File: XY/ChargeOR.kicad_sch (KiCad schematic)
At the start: 8 parts, among them U13 LTC4376CDHD_PBF, U9 SI3865DDV-T1-GE3

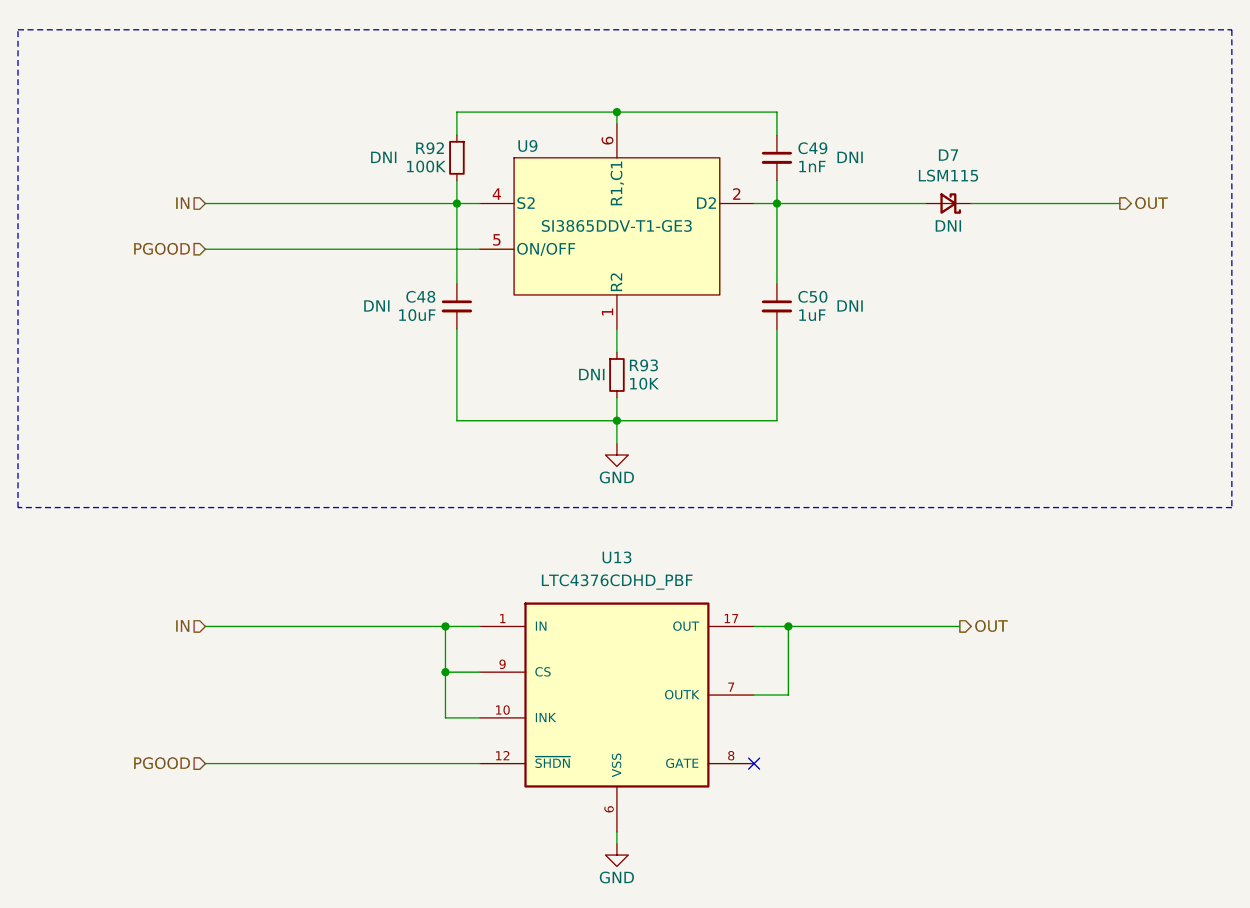
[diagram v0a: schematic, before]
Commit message: Updated XY boards
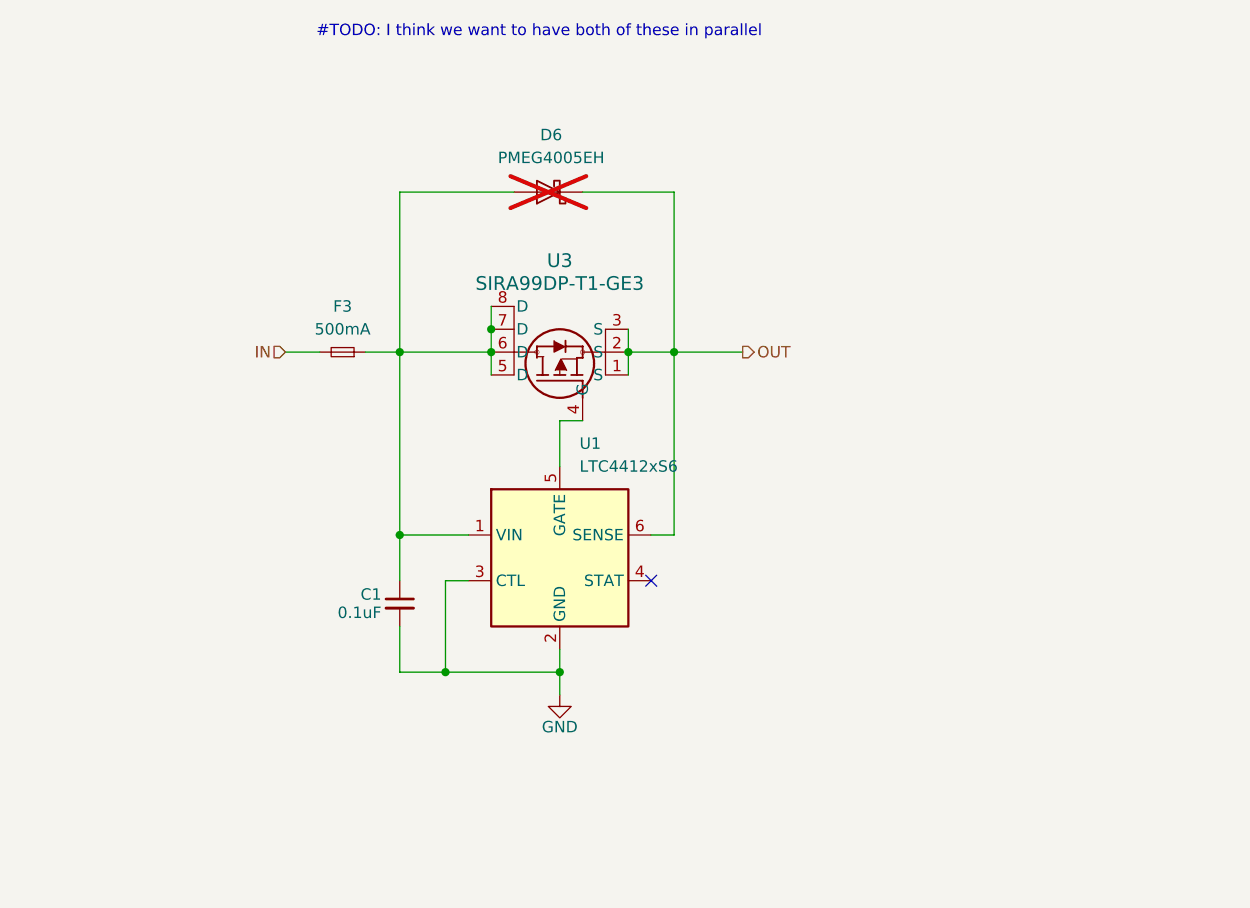
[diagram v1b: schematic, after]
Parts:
- removed C48: 10uF, Capacitor_SMD:C_1206_3216Metric, symbol Device:C_Small
- removed C49: 1nF, Capacitor_SMD:C_0603_1608Metric, symbol Device:C_Small
- removed C50: 1uF, Capacitor_SMD:C_1206_3216Metric, symbol Device:C_Small
- removed D7: LSM115, SolarPanels:DO-214BA_MCH, symbol Device:D_Schottky_Small
- removed R92: 100K, Resistor_SMD:R_0603_1608Metric, symbol Device:R_Small
- removed R93: 10K, Resistor_SMD:R_0603_1608Metric, symbol Device:R_Small
- removed U13: LTC4376CDHD_PBF, Package_DFN_QFN:DFN-16-1EP_4x5mm_P0.5mm_EP2.44x4.34mm, symbol SolarPanels:LTC4376CDHD_PBF
- removed U9: SI3865DDV-T1-GE3, Package_TO_SOT_SMD:SOT-23-6, symbol SolarPanels:SI3865DDV-T1-GE3
- added C1: 0.1uF, Capacitor_SMD:C_0603_1608Metric, symbol Device:C_Small
- added D6: PMEG4005EH, Diode_SMD:D_SOD-123F, symbol Diode:PMEG4005EH
- added F3: 500mA, symbol Device:Fuse_Small
- added U1: LTC4412xS6, Package_TO_SOT_SMD:TSOT-23-6, symbol Power_Management:LTC4412xS6
- added U3: SIRA99DP-T1-GE3, SolarPanels:MOSFET_7DP-T1-GE3_VIS, symbol Argus-Misc:SIRA99DP-T1-GE3
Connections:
- net GND: now also C1.2, U1.2 (GND), U1.3 (CTL)
- net IN: now also F3.2
- net OUT: now also D6.1 (K), U1.6 (SENSE), U3.1 (S), U3.2 (S), U3.3 (S)
- new net: C1.1, D6.2 (A), F3.1, U1.1 (VIN), U3.5 (D), U3.6 (D), U3.7 (D), U3.8 (D)
- new net: U1.5 (GATE), U3.4 (G)
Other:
- note added: "#TODO: I think we want to have both of these in parallel"
